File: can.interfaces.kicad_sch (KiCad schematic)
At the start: 6 parts, among them U2 TJA1051T, U3 TL431(2.5-36), U4 TCMT1107

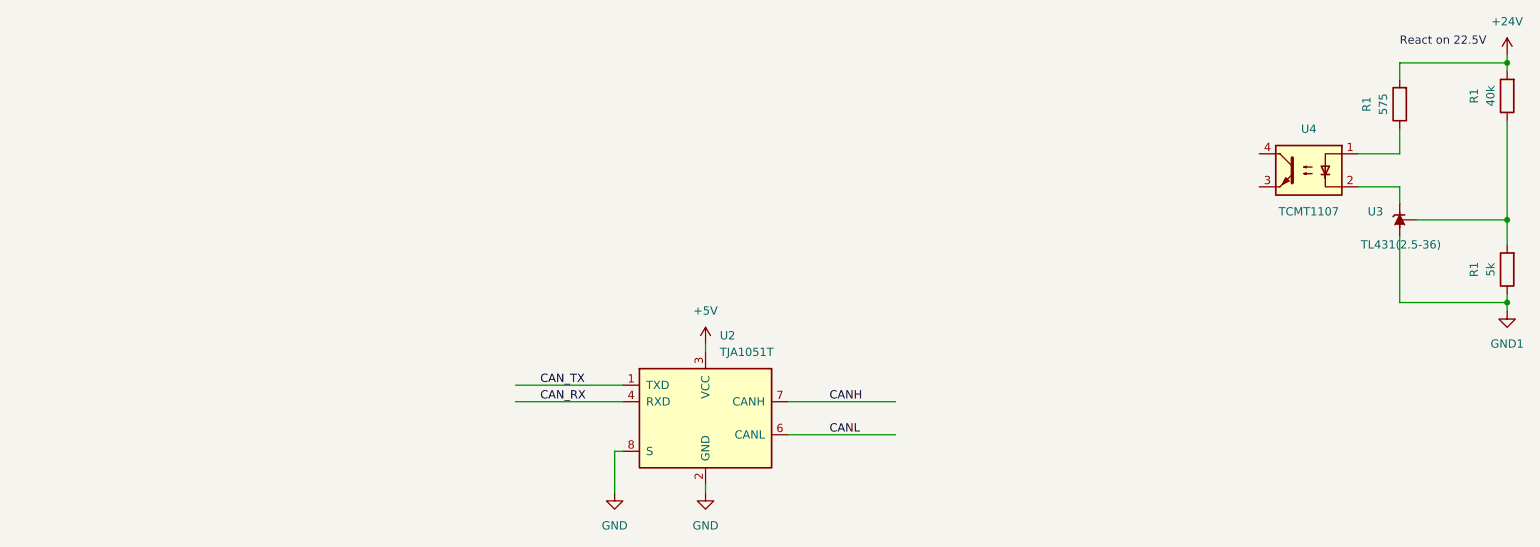
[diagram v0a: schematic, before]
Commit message: almost final schematics
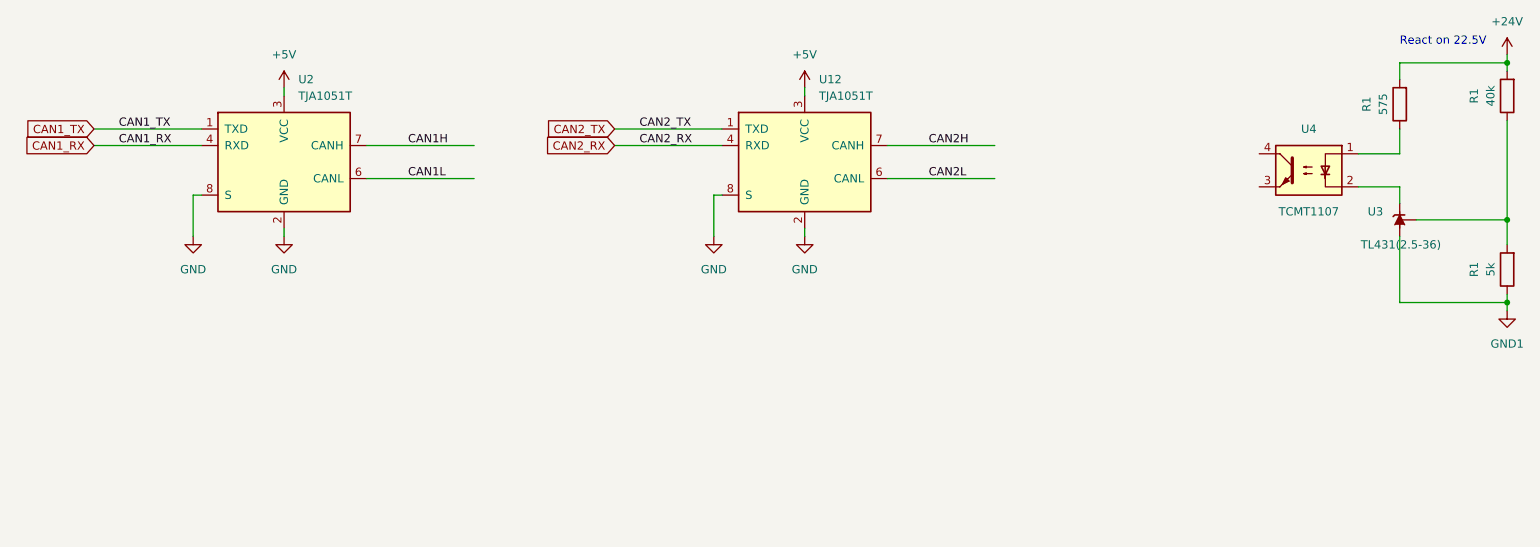
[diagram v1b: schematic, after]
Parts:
- added U12: TJA1051T, Package_SO:SOIC-8_3.9x4.9mm_P1.27mm, symbol Interface_CAN_LIN:TJA1051T
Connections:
- net +5V: now also U12.3 (VCC)
- net GND: now also U12.2 (GND), U12.8 (S)
- net CANH renamed CAN1H
- net CANL renamed CAN1L
- net CAN_RX renamed CAN1_RX
- net CAN_TX renamed CAN1_TX
- new net CAN2H: U12.7 (CANH)
- new net CAN2L: U12.6 (CANL)
- new net CAN2_RX: U12.4 (RXD)
- new net CAN2_TX: U12.1 (TXD)
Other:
- moved on the sheet: U2
